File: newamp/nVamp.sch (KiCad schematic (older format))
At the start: 8 parts, among them J1 CONN_01X02, J2 CONN_01X02, U1 TS912

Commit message: Update PCB to use AD8428 and AD4528 amps
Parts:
- removed J2: CONN_01X02, Pin_Headers:Pin_Header_Straight_1x02_Pitch2.54mm, symbol CONN_01X02
- removed R4: 1k, Resistors_SMD:R_0805_HandSoldering, symbol R
- removed R5: 10k, Resistors_SMD:R_0805_HandSoldering, symbol R
- removed U1: TS912, Housings_SOIC:SO-8_5.3x6.2mm_Pitch1.27mm, symbol TS912
- added C1: 100u, Capacitors_SMD:C_1210_HandSoldering, symbol C
- added C2, C3: 100n, Capacitors_SMD:C_0603_HandSoldering, symbol C_Small
- added J2: CONN_01X03, Pin_Headers:Pin_Header_Straight_1x03_Pitch2.54mm, symbol CONN_01X03
- added J3: CONN_01X02, Pin_Headers:Pin_Header_Straight_1x02_Pitch2.54mm, symbol CONN_01X02
- added U1: AD8428, Housings_SOIC:SOIC-8_3.9x4.9mm_Pitch1.27mm, symbol AD8428
- added U2: ADA4528, Housings_SSOP:TSSOP-8_3x3mm_Pitch0.65mm, symbol ADA4528
- R1: value 0 -> 15k
- R3: value 1k -> 100k
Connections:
- net labels added: VDD, VEE
- net labels removed: +3.3V, FB, GNDPWR
- wire segments 16 -> 9
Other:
- note removed: "Opamp TBD\n"
- note removed: "Seebeck Effect\nResistor\n"

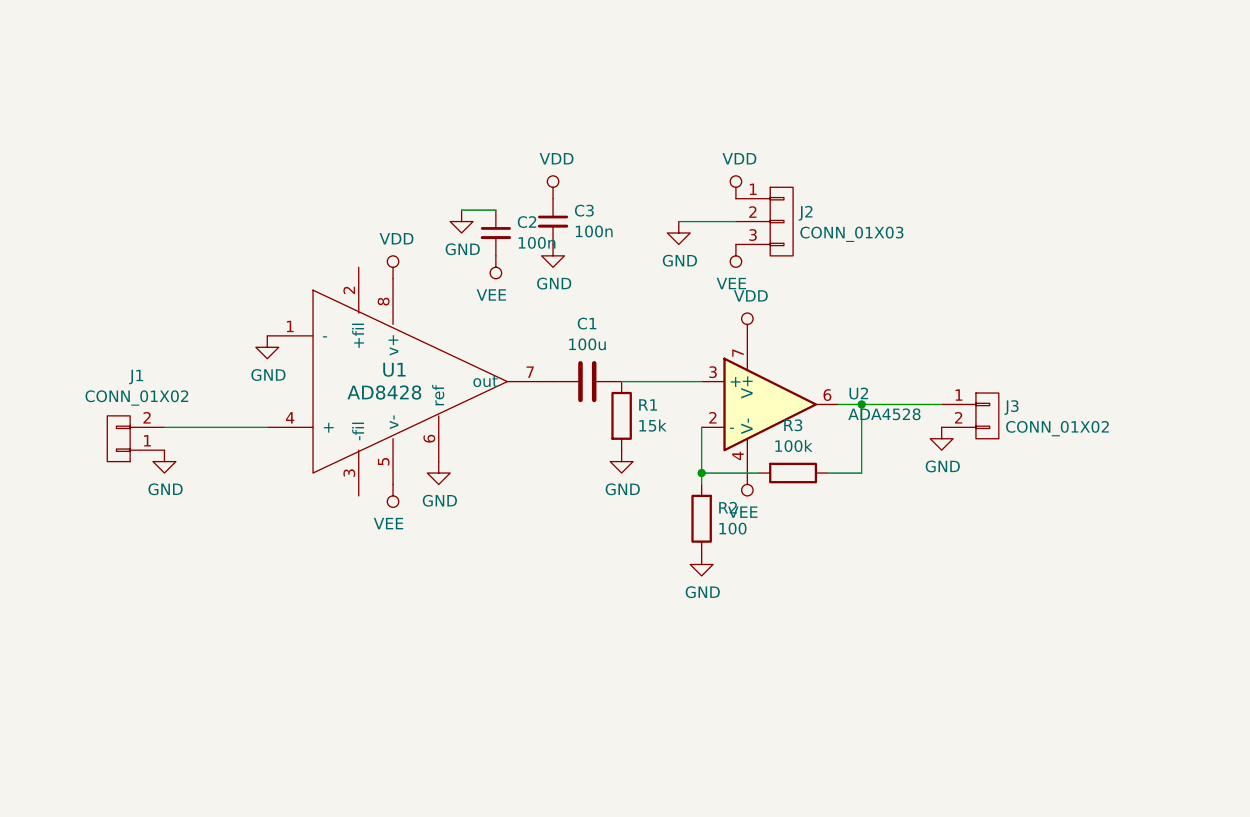
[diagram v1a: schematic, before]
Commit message: Pretty up schematics
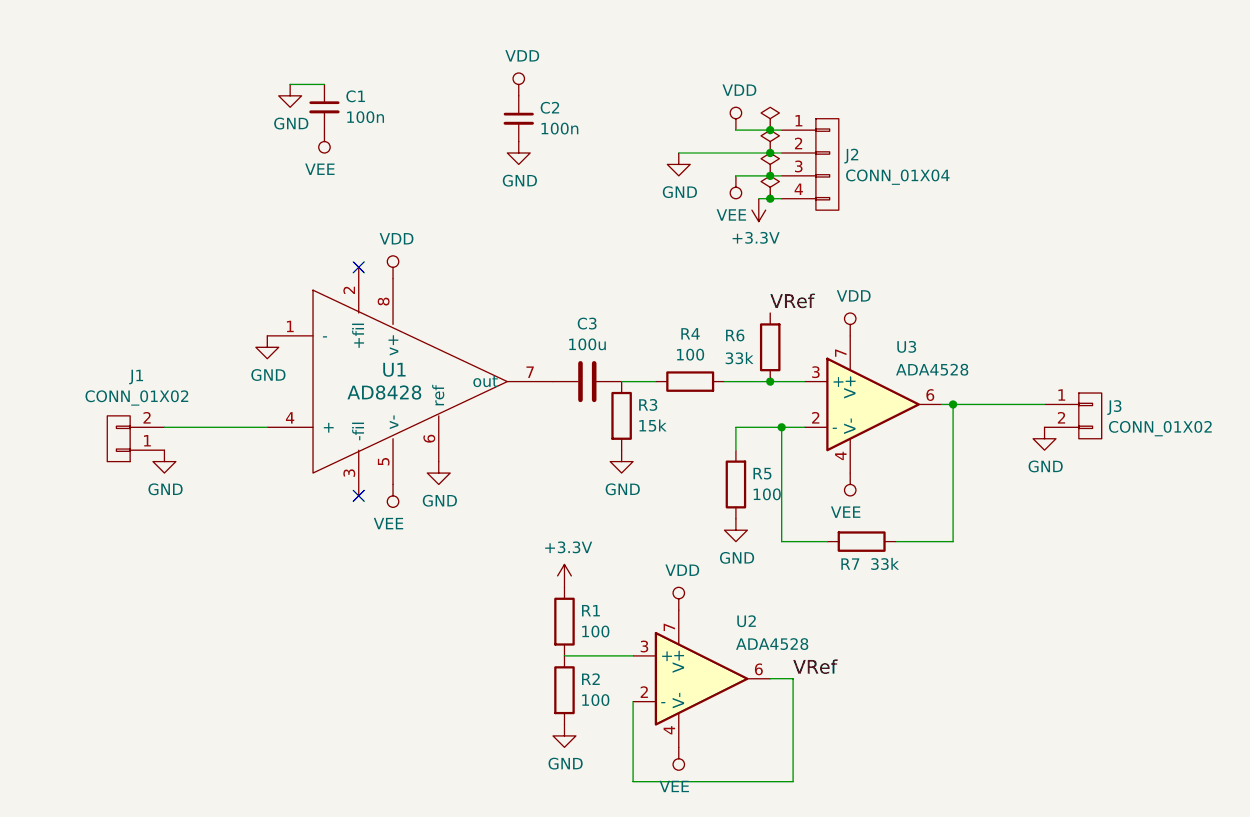
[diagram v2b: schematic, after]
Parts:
- removed J2: CONN_01X03, Pin_Headers:Pin_Header_Straight_1x03_Pitch2.54mm, symbol CONN_01X03
- removed R3: 100k, Resistors_SMD:R_0805_HandSoldering, symbol R
- added J2: CONN_01X04, symbol CONN_01X04
- added R1, R4, R5: 100, symbol R
- added R6, R7: 33k, symbol R
- added U2: ADA4528, Housings_SSOP:TSSOP-8_3x3mm_Pitch0.65mm, symbol ADA4528
- R2: footprint Resistors_SMD:R_0805_HandSoldering -> (none)
- renumbered C2 to C1, C3 to C2, C1 to C3, R1 to R3, U2 to U3
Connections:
- net GND: now also R2.2, J2.2 (P2), R5.1; no longer R2.1
- net VDD: now also J2.1 (P1), U2.7 (V+)
- net VEE: now also J2.3 (P3), U2.4 (V-)
- net at U3.2 (-): now also R5.2, R7.2; no longer R2.2
- net at C3.1, R3.1: now also R4.1; no longer U3.3 (+)
- net at J3.1 (P1), U3.6: now also R7.1
- new net: R4.2, R6.1, U3.3 (+)
- new net: R1.2, R2.1, U2.3 (+)
- new net +3V3: J2.4 (P4), R1.1
- new net VRef: R6.2, U2.2 (-), U2.6
- no-connect marks 0 -> 2
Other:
- moved on the sheet: C1, C2, J3, U3
